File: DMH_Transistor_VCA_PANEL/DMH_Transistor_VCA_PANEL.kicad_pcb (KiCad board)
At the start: 2 copper layers, 50 x 200 mm, 19 parts, among them J0 Panel_GND_Solder_Wire_Pad

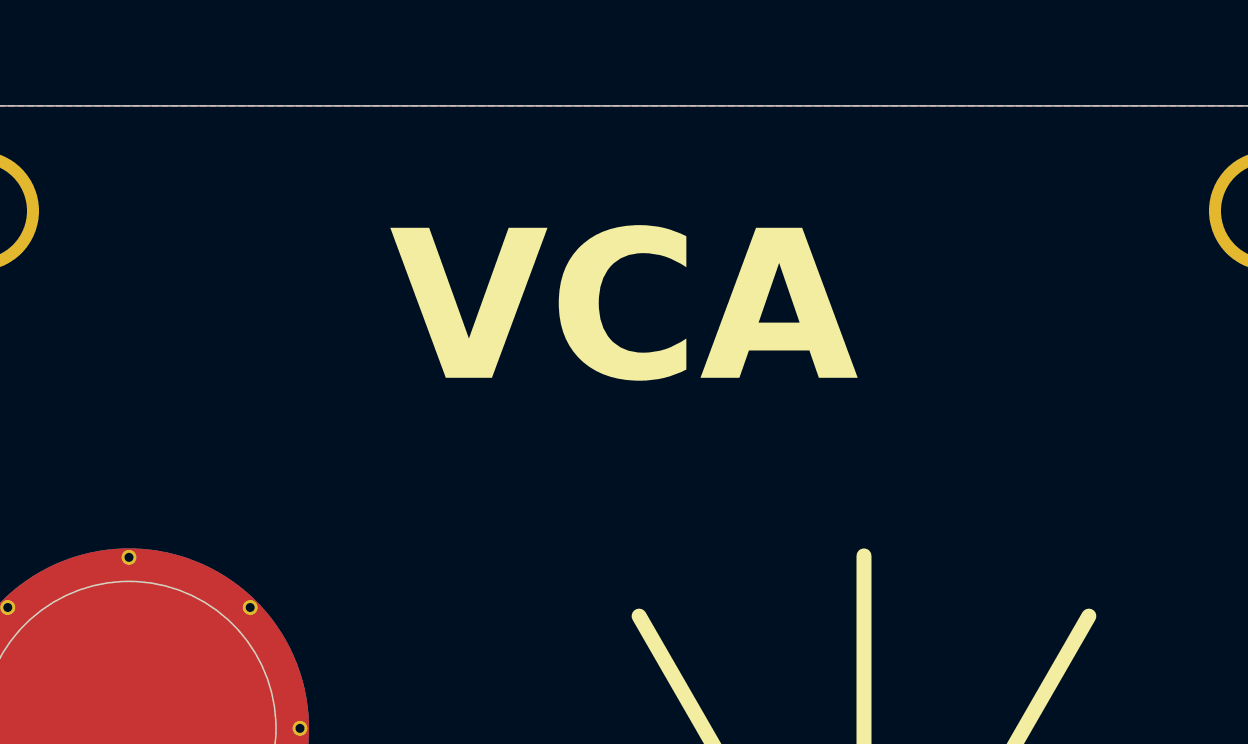
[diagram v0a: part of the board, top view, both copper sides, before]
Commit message: Finished schematic
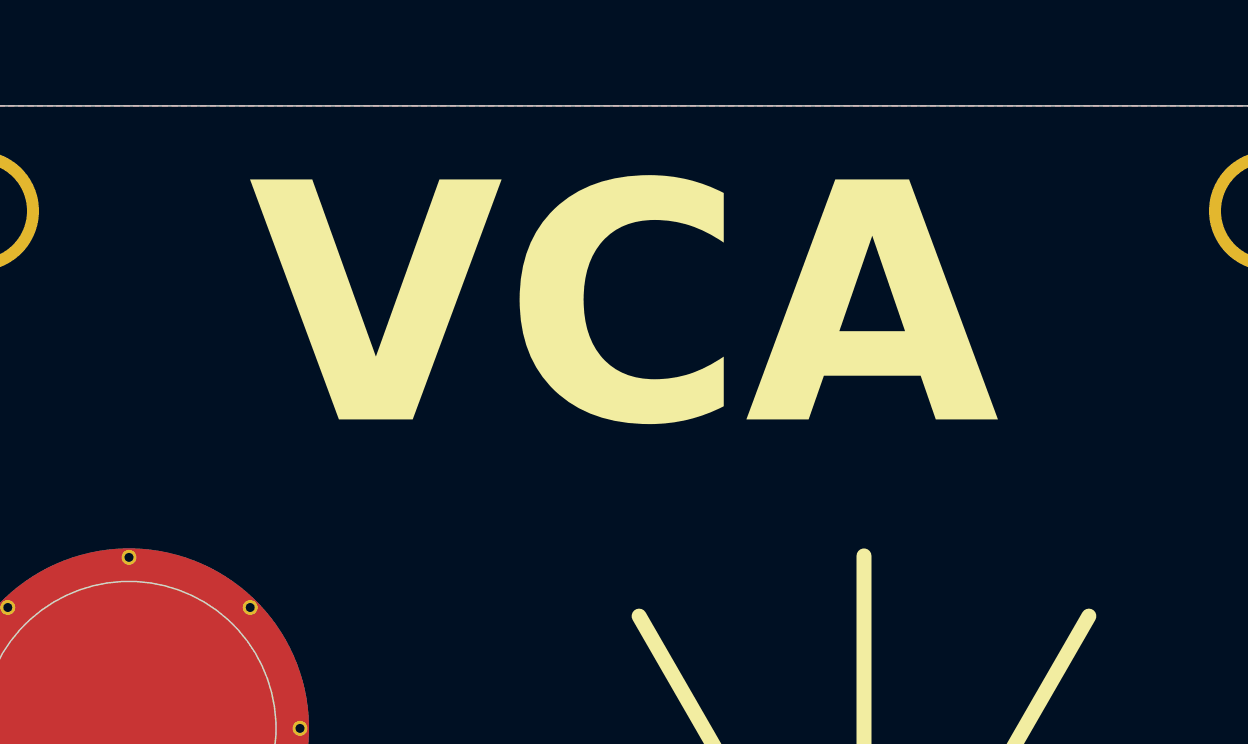
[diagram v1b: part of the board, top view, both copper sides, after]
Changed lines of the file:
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@@
 			(font
 				(face "Nulshock Rg")
-				(size 5 5)
+				(size 8 8)
 				(thickness 0.8)
 				(bold yes)
@@
 			(polygon
 				(pts
-					(xy 67.904745 38.032431) (xy 68.042519 38.2864) (xy 68.207021 38.495752) (xy 68.399395 38.661131)
-					(xy 68.620789 38.78318) (xy 68.872348 38.862542) (xy 69.155218 38.899859) (xy 69.27739 38.903157)
-					(xy 69.574662 38.882478) (xy 69.838057 38.820011) (xy 70.069476 38.715114) (xy 70.270819 38.567144)
-					(xy 70.443987 38.375459) (xy 70.590881 38.139414) (xy 70.642707 38.032431) (xy 72.336531 34.268649)
-					(xy 72.413468 34.057379) (xy 70.935799 34.057379) (xy 70.879623 34.225907) (xy 69.480111 37.506088)
-					(xy 69.283496 37.653855) (xy 69.080774 37.506088) (xy 67.666608 34.225907) (xy 67.61776 34.057379)
-					(xy 66.11933 34.057379) (xy 66.196266 34.268649)
+					(xy 63.647593 38.801891) (xy 63.868032 39.20824) (xy 64.131234 39.543203) (xy 64.439033 39.80781)
+					(xy 64.793263 40.003088) (xy 65.195757 40.130067) (xy 65.648349 40.189774) (xy 65.843824 40.195052)
+					(xy 66.31946 40.161965) (xy 66.740892 40.062018) (xy 67.111162 39.894183) (xy 67.433311 39.657431)
+					(xy 67.71038 39.350734) (xy 67.94541 38.973062) (xy 68.028332 38.801891) (xy 70.738451 32.779839)
+					(xy 70.861549 32.441807) (xy 68.497279 32.441807) (xy 68.407397 32.711451) (xy 66.168179 37.959741)
+					(xy 65.853594 38.196168) (xy 65.52924 37.959741) (xy 63.266574 32.711451) (xy 63.188416 32.441807)
+					(xy 60.790928 32.441807) (xy 60.914027 32.779839)
 				)
 			)
 			(polygon
 				(pts
-					(xy 77.196964 37.579361) (xy 74.71912 37.579361) (xy 74.445674 37.5596) (xy 74.180981 37.491641)
-					(xy 73.962685 37.380219) (xy 73.766573 37.209333) (xy 73.617966 37.003456) (xy 73.51824 36.765021)
-					(xy 73.474774 36.502973) (xy 73.473482 36.448517) (xy 73.503956 36.185317) (xy 73.590923 35.941842)
-					(xy 73.7277 35.727383) (xy 73.822749 35.624197) (xy 74.034928 35.466729) (xy 74.271818 35.368069)
-					(xy 74.530274 35.32023) (xy 74.71912 35.311566) (xy 77.196964 35.311566) (xy 77.196964 34.057379)
-					(xy 74.71912 34.057379) (xy 74.442017 34.068365) (xy 74.182759 34.100618) (xy 73.940761 34.153077)
-					(xy 73.66164 34.245455) (xy 73.407423 34.365684) (xy 73.176965 34.511695) (xy 72.96912 34.68142)
-					(xy 72.762549 34.898539) (xy 72.584298 35.141469) (xy 72.437106 35.407219) (xy 72.343556 35.634239)
-					(xy 72.273041 35.872418) (xy 72.226961 36.120225) (xy 72.20672 36.376128) (xy 72.205861 36.441189)
-					(xy 72.22245 36.733118) (xy 72.270947 37.013346) (xy 72.349453 37.279833) (xy 72.456067 37.530539)
-					(xy 72.588888 37.763423) (xy 72.746016 37.976444) (xy 72.815247 38.055635) (xy 73.032464 38.265052)
-					(xy 73.278219 38.44512) (xy 73.495915 38.566353) (xy 73.73281 38.665905) (xy 73.989318 38.742487)
-					(xy 74.265855 38.794812) (xy 74.562834 38.821592) (xy 74.71912 38.825) (xy 77.196964 38.825)
+					(xy 78.515143 38.076978) (xy 74.550593 38.076978) (xy 74.11308 38.045361) (xy 73.689571 37.936626)
+					(xy 73.340297 37.758351) (xy 73.026518 37.484933) (xy 72.788746 37.15553) (xy 72.629184 36.774034)
+					(xy 72.55964 36.354757) (xy 72.557572 36.267627) (xy 72.606331 35.846507) (xy 72.745478 35.456947)
+					(xy 72.96432 35.113813) (xy 73.116399 34.948715) (xy 73.455885 34.696766) (xy 73.834909 34.538911)
+					(xy 74.24844 34.462369) (xy 74.550593 34.448506) (xy 78.515143 34.448506) (xy 78.515143 32.441807)
+					(xy 74.550593 32.441807) (xy 74.107228 32.459385) (xy 73.692416 32.510989) (xy 73.305218 32.594924)
+					(xy 72.858624 32.742729) (xy 72.451878 32.935094) (xy 72.083146 33.168712) (xy 71.750593 33.440272)
+					(xy 71.420079 33.787663) (xy 71.134877 34.176351) (xy 70.899371 34.601551) (xy 70.749691 34.964782)
+					(xy 70.636866 35.345869) (xy 70.563138 35.74236) (xy 70.530753 36.151805) (xy 70.529379 36.255903)
+					(xy 70.55592 36.722989) (xy 70.633516 37.171354) (xy 70.759126 37.597733) (xy 70.929708 37.998862)
+					(xy 71.142222 38.371476) (xy 71.393627 38.712311) (xy 71.504397 38.839016) (xy 71.851943 39.174083)
+					(xy 72.245151 39.462193) (xy 72.593465 39.656165) (xy 72.972497 39.815448) (xy 73.38291 39.93798)
+					(xy 73.825368 40.0217) (xy 74.300536 40.064547) (xy 74.550593 40.07) (xy 78.515143 40.07)
 				)
 			)
 			(polygon
 				(pts
-					(xy 80.838607 33.982587) (xy 81.118933 34.020535) (xy 81.368787 34.100873) (xy 81.589146 34.223854)
-					(xy 81.78099 34.389729) (xy 81.945296 34.59875) (xy 82.083042 34.851168) (xy 83.791521 38.610066)
-					(xy 83.868457 38.825) (xy 82.439637 38.825) (xy 82.384682 38.660136) (xy 82.131891 38.07151) (xy 79.331646 38.07151)
-					(xy 79.087404 38.652808) (xy 79.037334 38.825) (xy 77.574319 38.825) (xy 77.651256 38.610066) (xy 78.364959 37.027372)
-					(xy 79.794487 37.027372) (xy 81.670272 37.027372) (xy 80.942428 35.339654) (xy 80.933949 35.320902)
-					(xy 80.725052 35.193108) (xy 80.717174 35.193213) (xy 80.515003 35.339654) (xy 79.794487 37.027372)
-					(xy 78.364959 37.027372) (xy 79.346301 34.851168) (xy 79.398116 34.744977) (xy 79.544948 34.509948)
-					(xy 79.718189 34.318216) (xy 79.919963 34.169528) (xy 80.152394 34.063635) (xy 80.417607 34.000283)
-					(xy 80.717725 33.979221)
+					(xy 84.341772 32.32214) (xy 84.790294 32.382856) (xy 85.19006 32.511397) (xy 85.542635 32.708167)
+					(xy 85.849585 32.973567) (xy 86.112474 33.308) (xy 86.332868 33.71187) (xy 89.066434 39.726106)
+					(xy 89.189533 40.07) (xy 86.90342 40.07) (xy 86.815492 39.806217) (xy 86.411026 38.864417) (xy 81.930635 38.864417)
+					(xy 81.539847 39.794494) (xy 81.459735 40.07) (xy 79.118912 40.07) (xy 79.24201 39.726106) (xy 80.383936 37.193796)
+					(xy 82.67118 37.193796) (xy 85.672436 37.193796) (xy 84.507886 34.493447) (xy 84.49432 34.463444)
+					(xy 84.160084 34.258974) (xy 84.14748 34.259142) (xy 83.824006 34.493447) (xy 82.67118 37.193796)
+					(xy 80.383936 37.193796) (xy 81.954083 33.71187) (xy 82.036986 33.541964) (xy 82.271918 33.165917)
+					(xy 82.549104 32.859145) (xy 82.871942 32.621246) (xy 83.243832 32.451816) (xy 83.668171 32.350453)
+					(xy 84.14836 32.316755)
 				)
 			)
@@
 		)
 	)
-	(dimension
-		(type aligned)
-		(layer "Cmts.User")
-		(pts
-			(xy 50 108.125) (xy 50 130)
-		)
-		(height 0)
-		(gr_text "21.8750 mm"
-			(at 48.85 119.0625 90)
-			(layer "Cmts.User")
-			(effects
-				(font
-					(size 1 1)
-					(thickness 0.15)
-				)
-			)
-		)
-		(format
-			(prefix "")
-			(suffix "")
-			(units 3)
-			(units_format 1)
-			(precision 4)
-		)
-		(style
-			(thickness 0.1)
-			(arrow_length 1.27)
-			(text_position_mode 0)
-			(extension_height 0.58642)
-			(extension_offset 0.5) keep_text_aligned)
-	)
-	(dimension
-		(type aligned)
-		(layer "Cmts.User")
-		(pts
-			(xy 50 108.125) (xy 50 86.25)
-		)
-		(height 0)
-		(gr_text "21.8750 mm"
-			(at 48.85 97.1875 90)
-			(layer "Cmts.User")
-			(effects
-				(font
-					(size 1 1)
-					(thickness 0.15)
-				)
-			)
-		)
-		(format
-			(prefix "")
-			(suffix "")
-			(units 3)
-			(units_format 1)
-			(precision 4)
-		)
-		(style
-			(thickness 0.1)
-			(arrow_length 1.27)
-			(text_position_mode 0)
-			(extension_height 0.58642)
-			(extension_offset 0.5) keep_text_aligned)
-	)
 	(zone
